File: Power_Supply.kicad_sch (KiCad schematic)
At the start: 12 parts, among them U2 R-785.0-1.0

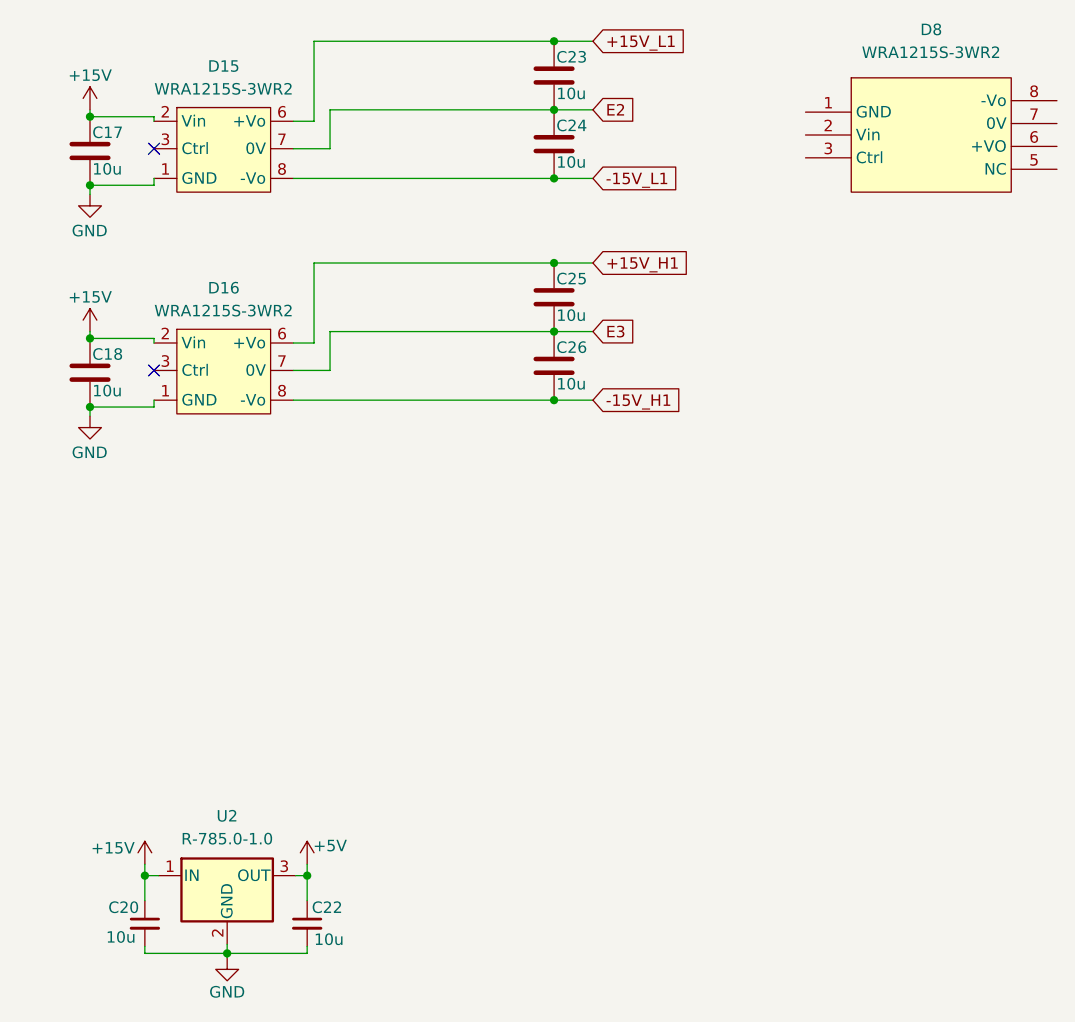
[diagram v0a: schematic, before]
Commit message: Развел все дорожки
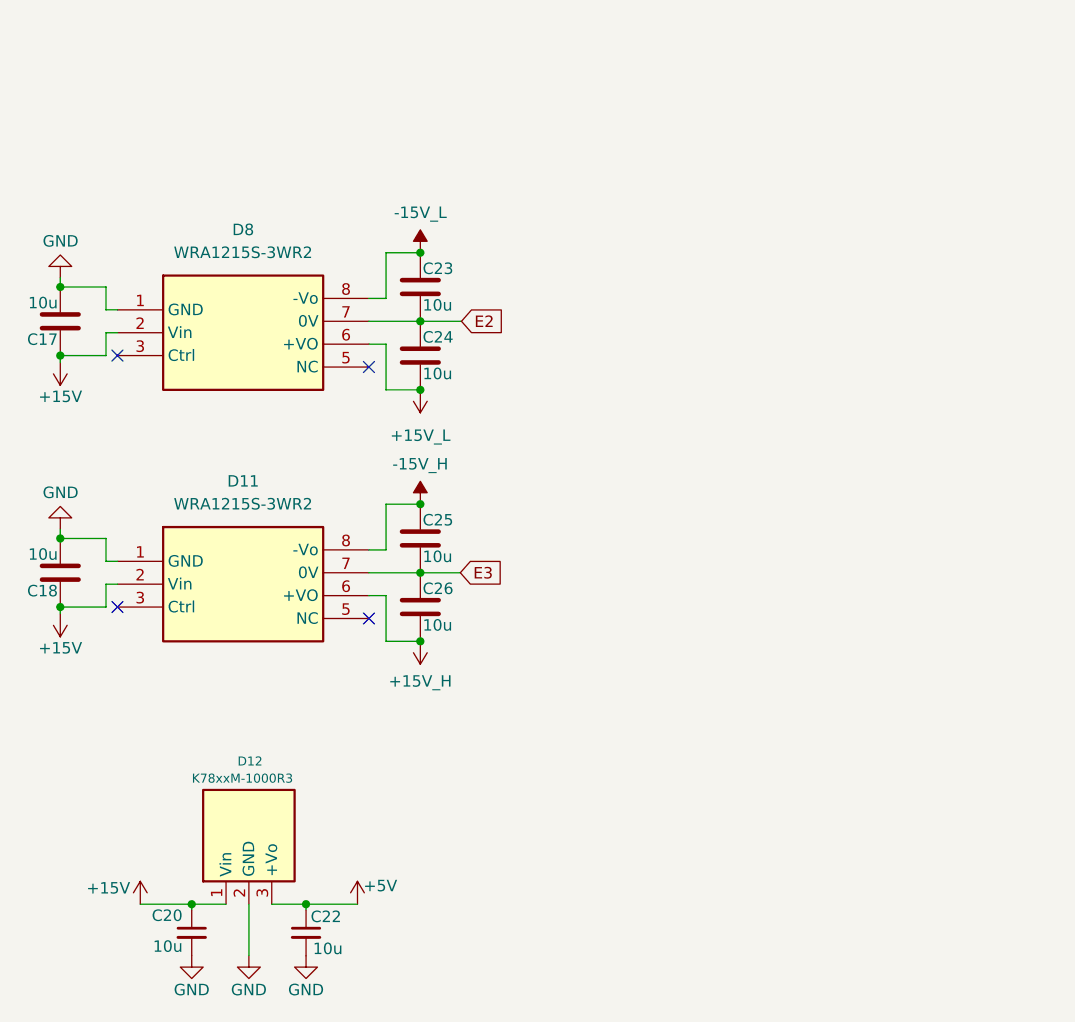
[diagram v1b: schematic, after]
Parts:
- removed D15, D16: WRA1215S-3WR2, Mornsun:WRA1215S-3WR2, symbol Morsun:WRA1215S-3WR2
- removed U2: R-785.0-1.0, Converter_DCDC:Converter_DCDC_RECOM_R-78E-0.5_THT, symbol Regulator_Switching:R-783.3-1.0
- added D11: WRA1215S-3WR2, Mornsun:WRA_S-3WR2, symbol Mornsun:WRA_S-3WR2
- added D12: K78xxM-1000R3, Mornsun:K78xx-1000R3, symbol Mornsun:K78xxM-1000R3 ÕýÊä³ö
- D8: footprint (none) -> Mornsun:WRA_S-3WR2
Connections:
- net +15V_L1 is gone; now on net -15V_L: C23.1
- net -15V_L1 is gone; now on net +15V_L: C24.2
- net +15V: now also D8.2 (Vin), D11.2 (Vin), D12.1 (Vin)
- net +5V: now also D12.3 (+Vo)
- net E2: now also D8.7 (0V)
- net E3: now also D11.7 (0V)
- net GND: now also D8.1 (GND), D11.1 (GND), D12.2 (GND)
- net +15V_L: now reaches D8.6 (+VO)
- net -15V_L: now reaches D8.8 (-Vo)
- net +15V_H1 renamed -15V_H
- net -15V_H: now also D11.8 (-Vo)
- net -15V_H1 renamed +15V_H
- net +15V_H: now also D11.6 (+VO)
- no-connect marks 2 -> 4
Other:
- moved on the sheet: C17, C18, C20, C22, C23, C24, C25, C26
